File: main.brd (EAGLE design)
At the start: 76.2 x 63.5 mm, 49 parts, among them J1 PJ-036AH-SMT-TR, J3 1734510-1, U1 ATMEGA328P-AU, U2 DRV8833PWPR, U3 LS7366R-S, U4 LP38691DTX-5.0/NOPB, U5 FT232RL-REEL, Y1 16MHz, Y2 30MHz

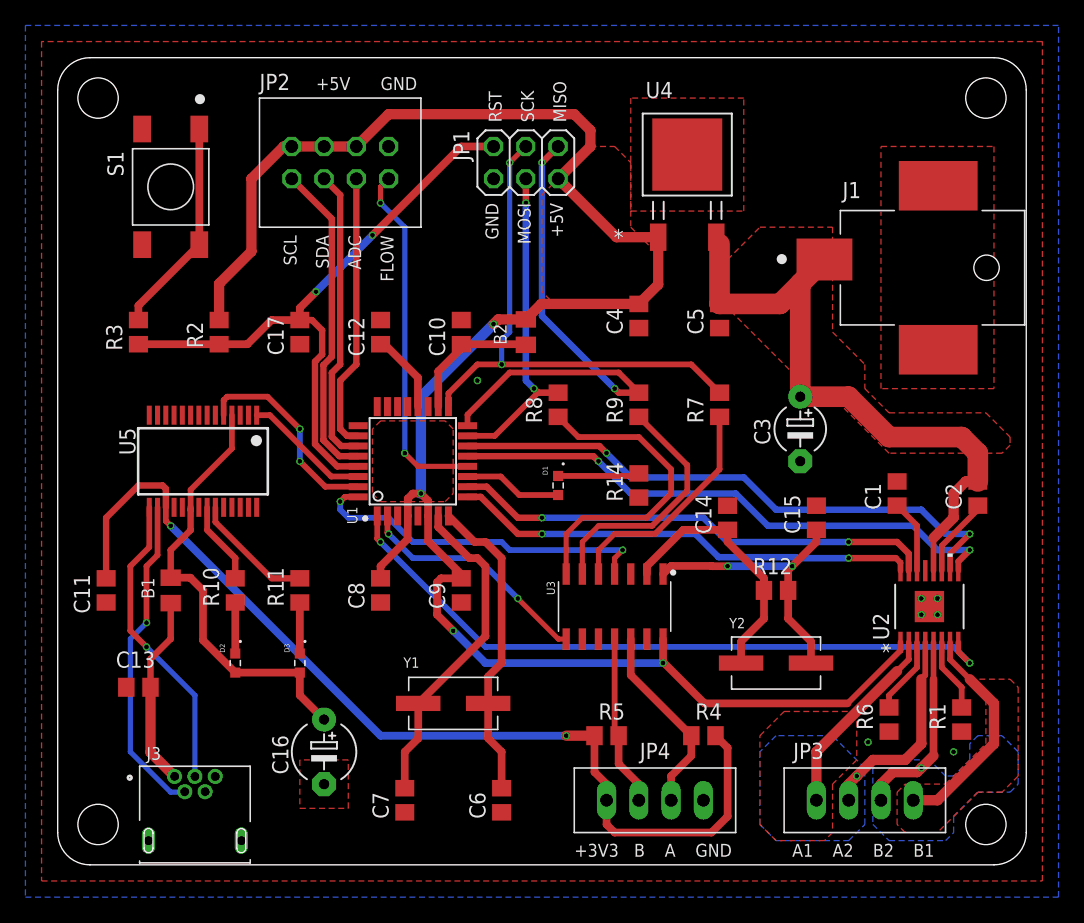
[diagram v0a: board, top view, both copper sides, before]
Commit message: Add files via upload
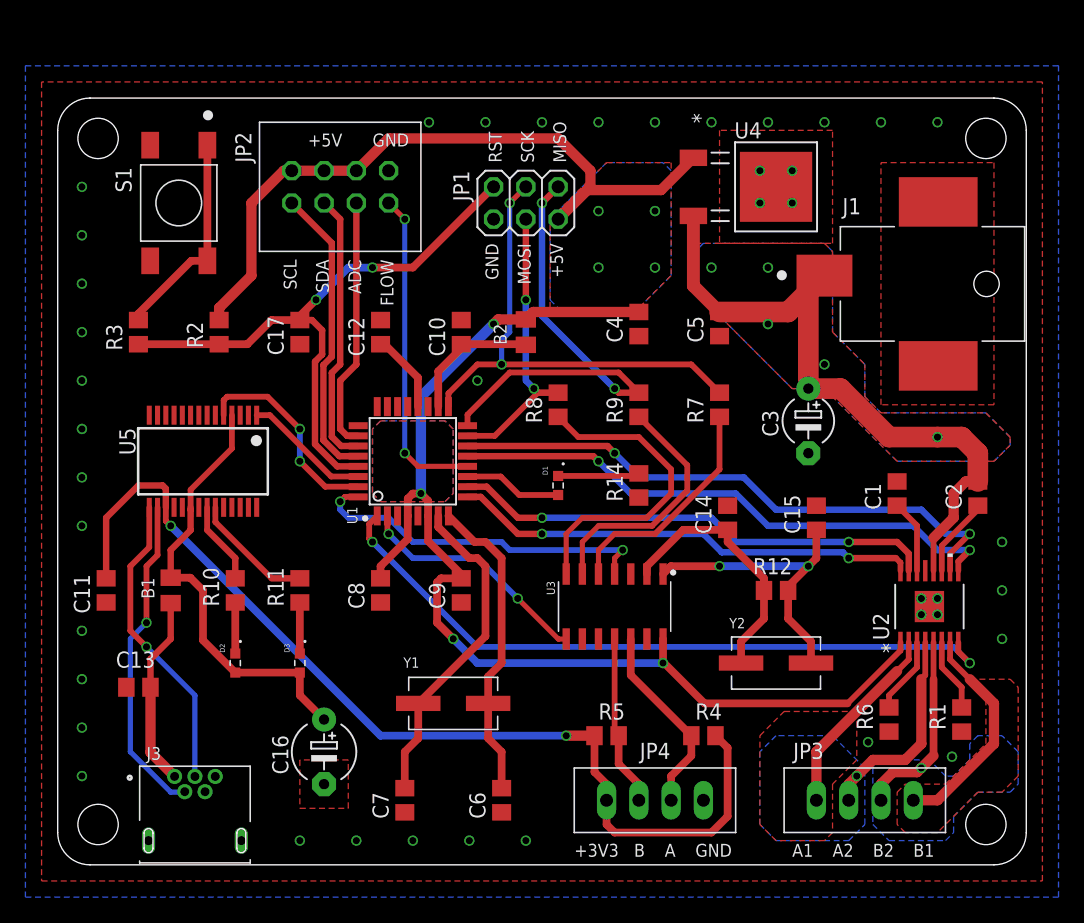
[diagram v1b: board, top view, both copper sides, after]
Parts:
- moved U4 7.43 mm to (56.5, 53.3), turned to 270 degrees
- moved JP1 3.17 mm to (36.8, 52.1)
- moved JP2 1.90 mm to (22.2, 53.3)
- moved S1 1.42 mm to (9.53, 52.1)
- moved J1 1.27 mm to (60.3, 46.4)
- moved C3 0.90 mm to (59.1, 34.9)
- moved C4 0.63 mm to (45.7, 42.5)
- moved C5 0.63 mm to (52.1, 42.5)
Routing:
- net +5V: track 154.3 -> 150.0 mm, vias 4 -> 8
- net MOSI: track 27.3 -> 24.2 mm
- net SCK: track 42.2 -> 39.0 mm
- net MISO: track 40.4 -> 37.2 mm
- net FLOW: track 28.0 -> 25.6 mm
- net SDA: track 23.5 -> 21.6 mm
- net SCL: track 25.4 -> 23.5 mm
- net ADC: track 21.8 -> 19.9 mm
- net !RESET!: track 50.3 -> 48.7 mm
- net FCKO: track 22.6 -> 23.8 mm
- net !FAULT!: track 54.5 -> 55.4 mm
- net VIN: track 53.7 -> 54.0 mm, vias 0 -> 5
- added copper zone on layer 16, net +5V
- added copper zone on layer 16, net VIN
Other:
- board size 76.2 x 63.5 mm -> 76.2 x 60.3 mm
